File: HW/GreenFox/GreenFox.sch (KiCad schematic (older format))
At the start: 29 parts, among them J1 USB_C_Receptacle_USB2.0, J2 Conn_02x05_Odd_Even, J3 Conn_01x14, J5 Conn_01x14, SW1 SW_Push, SW2 SW_Push, U1 LN1134-3.3V, U2 SRV05-4, U3 PIC32MM0256GPM036-IM2, Y1 Crystal_GND2, Y2 Crystal

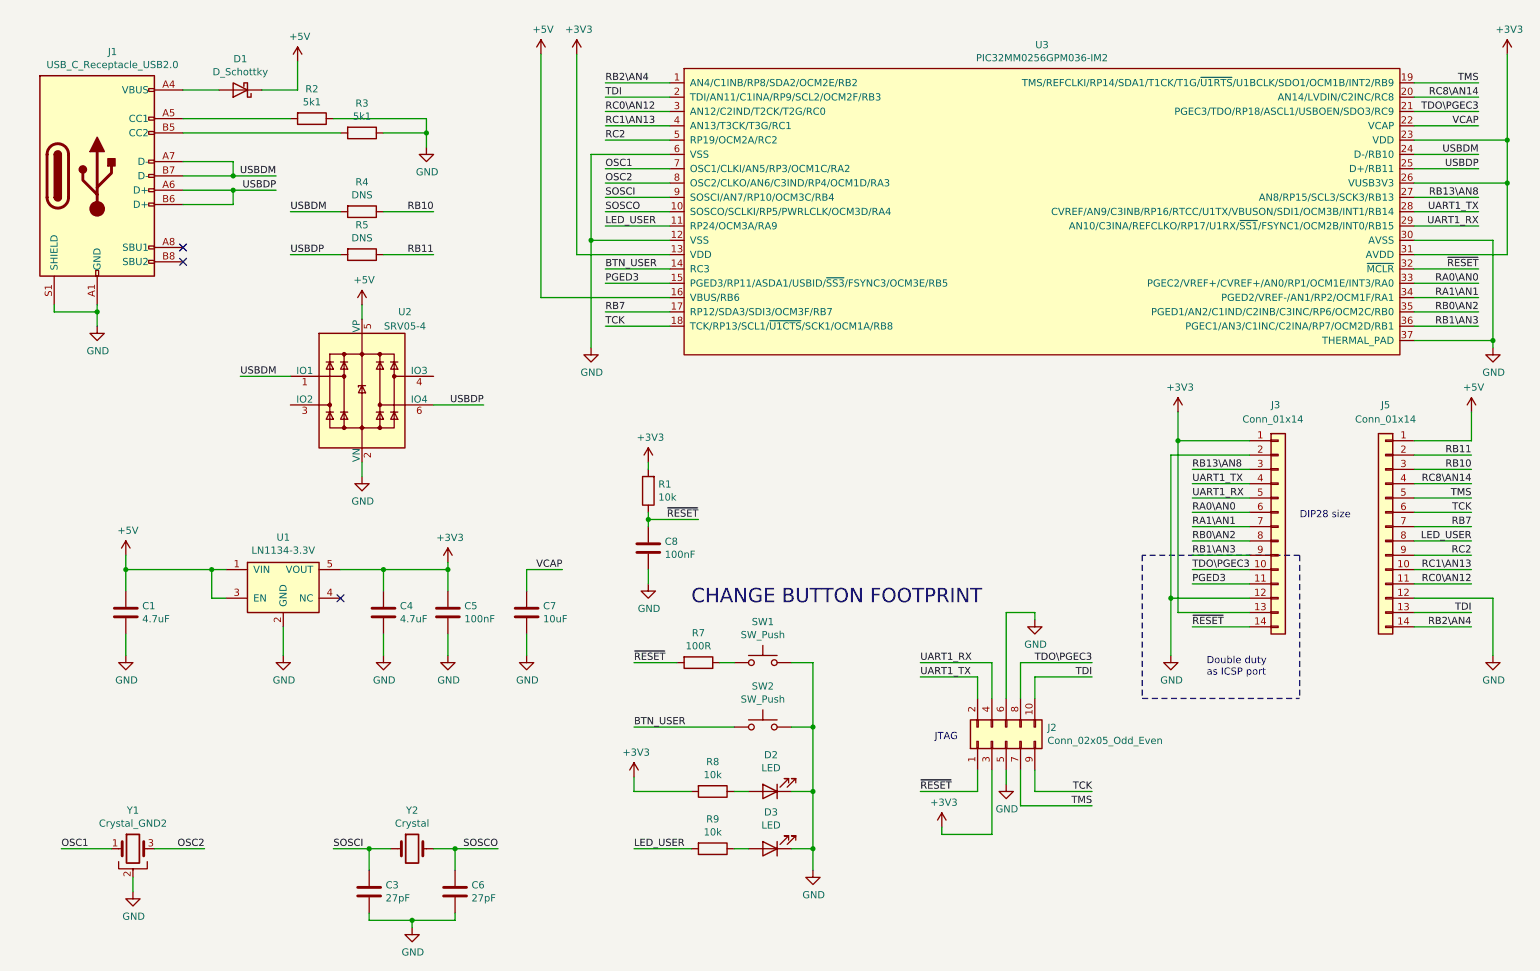
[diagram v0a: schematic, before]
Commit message: Finished board, added text, fiducials, logos, etc.
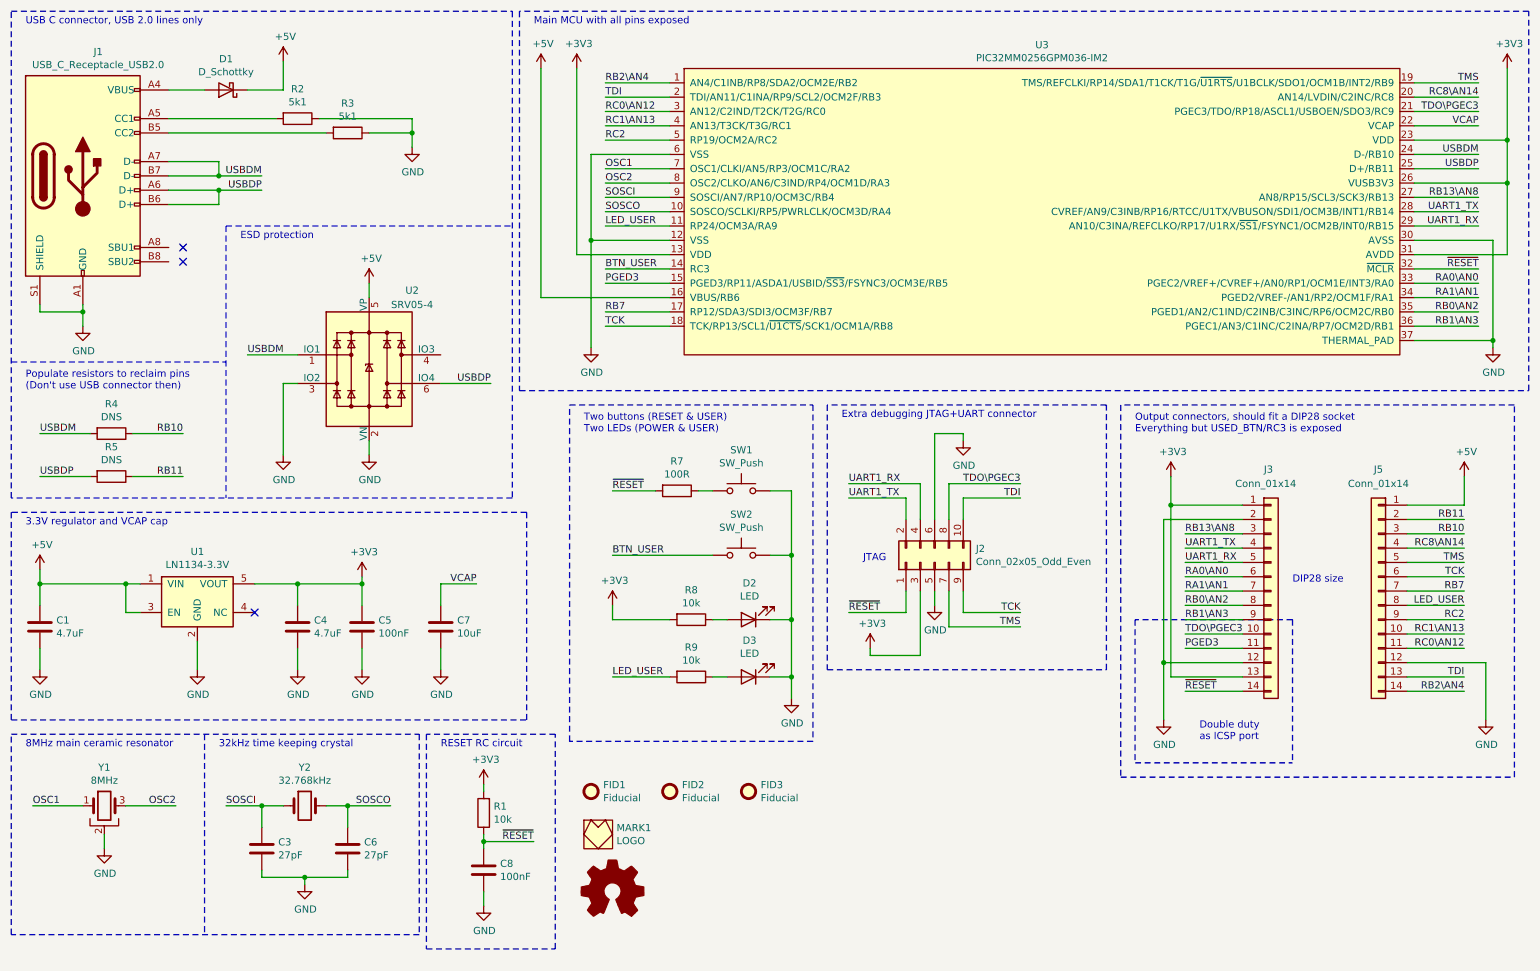
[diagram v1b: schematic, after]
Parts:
- added FID1, FID2, FID3: Fiducial, Fiducial:Fiducial_0.5mm_Mask1mm, symbol Mechanical:Fiducial
- added MARK1: LOGO, KiCAD library:FOX_LOGO_MASK, symbol Kicad_Library:LOGO
- Y1: value Crystal_GND2 -> 8MHz
- Y2: value Crystal -> 32.768kHz
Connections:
- net GND: now also U2.3 (IO2)
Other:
- note added: "3.3V regulator and VCAP cap"
- note added: "32kHz time keeping crystal"
- note added: "8MHz main ceramic resonator"
- note added: "ESD protection"
- note added: "Extra debugging JTAG+UART connector"
- note added: "Main MCU with all pins exposed"
- note added: "Output connectors, should fit a DIP28 socket\nEverything but USED_BTN/RC3 is exposed"
- note added: "Populate resistors to reclaim pins\n(Don't use USB connector then)"
- note added: "RESET RC circuit"
- note added: "Two buttons (RESET & USER)\nTwo LEDs (POWER & USER)"
- note added: "USB C connector, USB 2.0 lines only"
- note removed: "CHANGE BUTTON FOOTPRINT"
- moved on the sheet: C1, C3, C4, C5, C6, C7, C8, D1, D2, D3, J1, J2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
